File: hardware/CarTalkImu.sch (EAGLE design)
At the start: 35 parts, among them J4 1X10, J5 1X10, U1 LPS22HB, U3 MPU9250, U4 CAM-M8

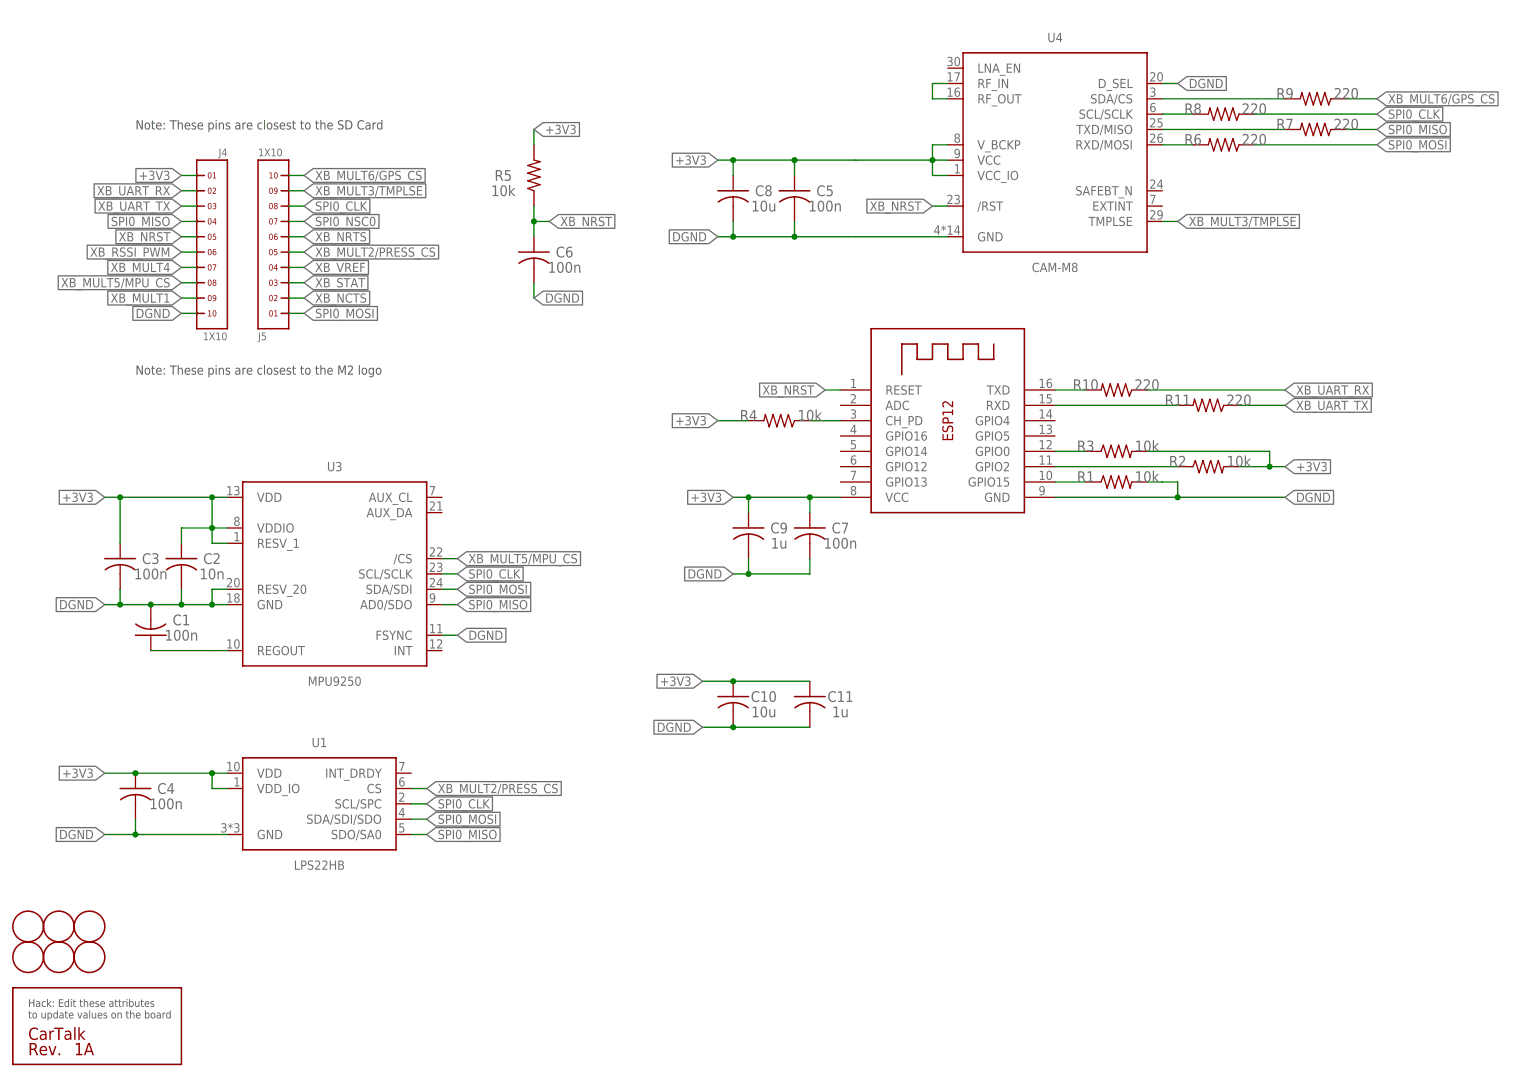
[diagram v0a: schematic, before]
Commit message: Re-finalized design and layout.
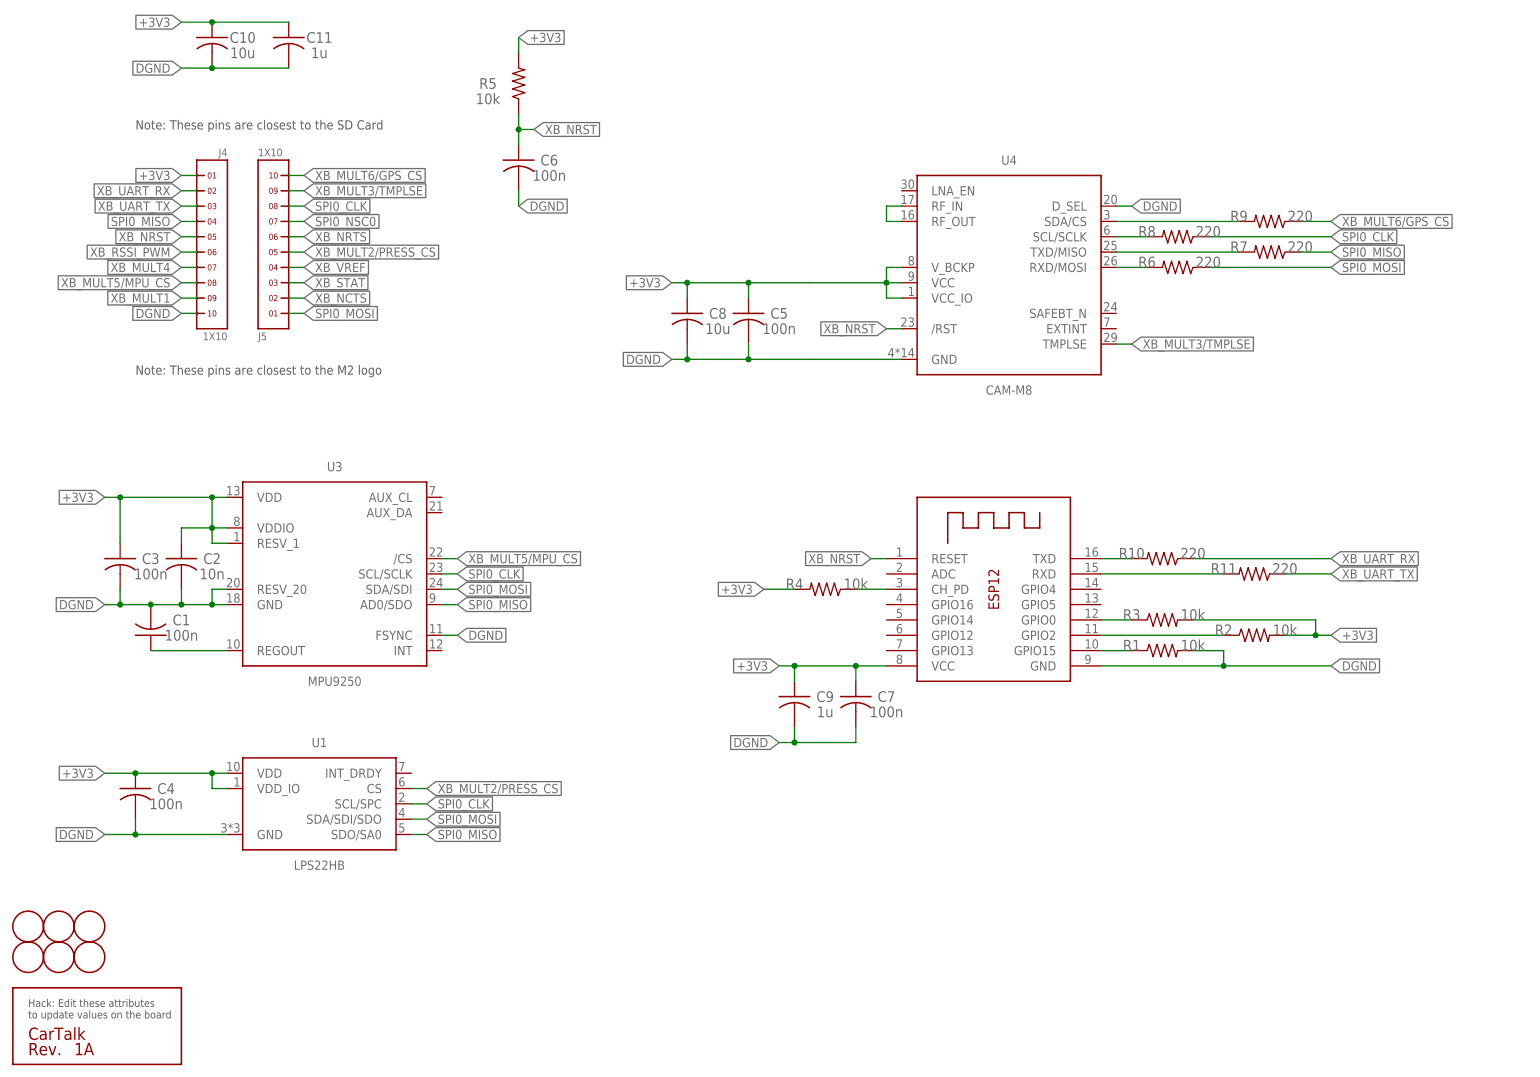
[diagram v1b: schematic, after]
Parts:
- X1: value (none) -> ESP-12
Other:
- moved on the sheet: C10, C11, C5, C6, C7, C8, C9, R1, R10, R11, R2, R3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
